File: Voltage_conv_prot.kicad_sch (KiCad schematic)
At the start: 6 parts, among them Q1 AO3400A, U6 MIC5504-3.3YM5-TR

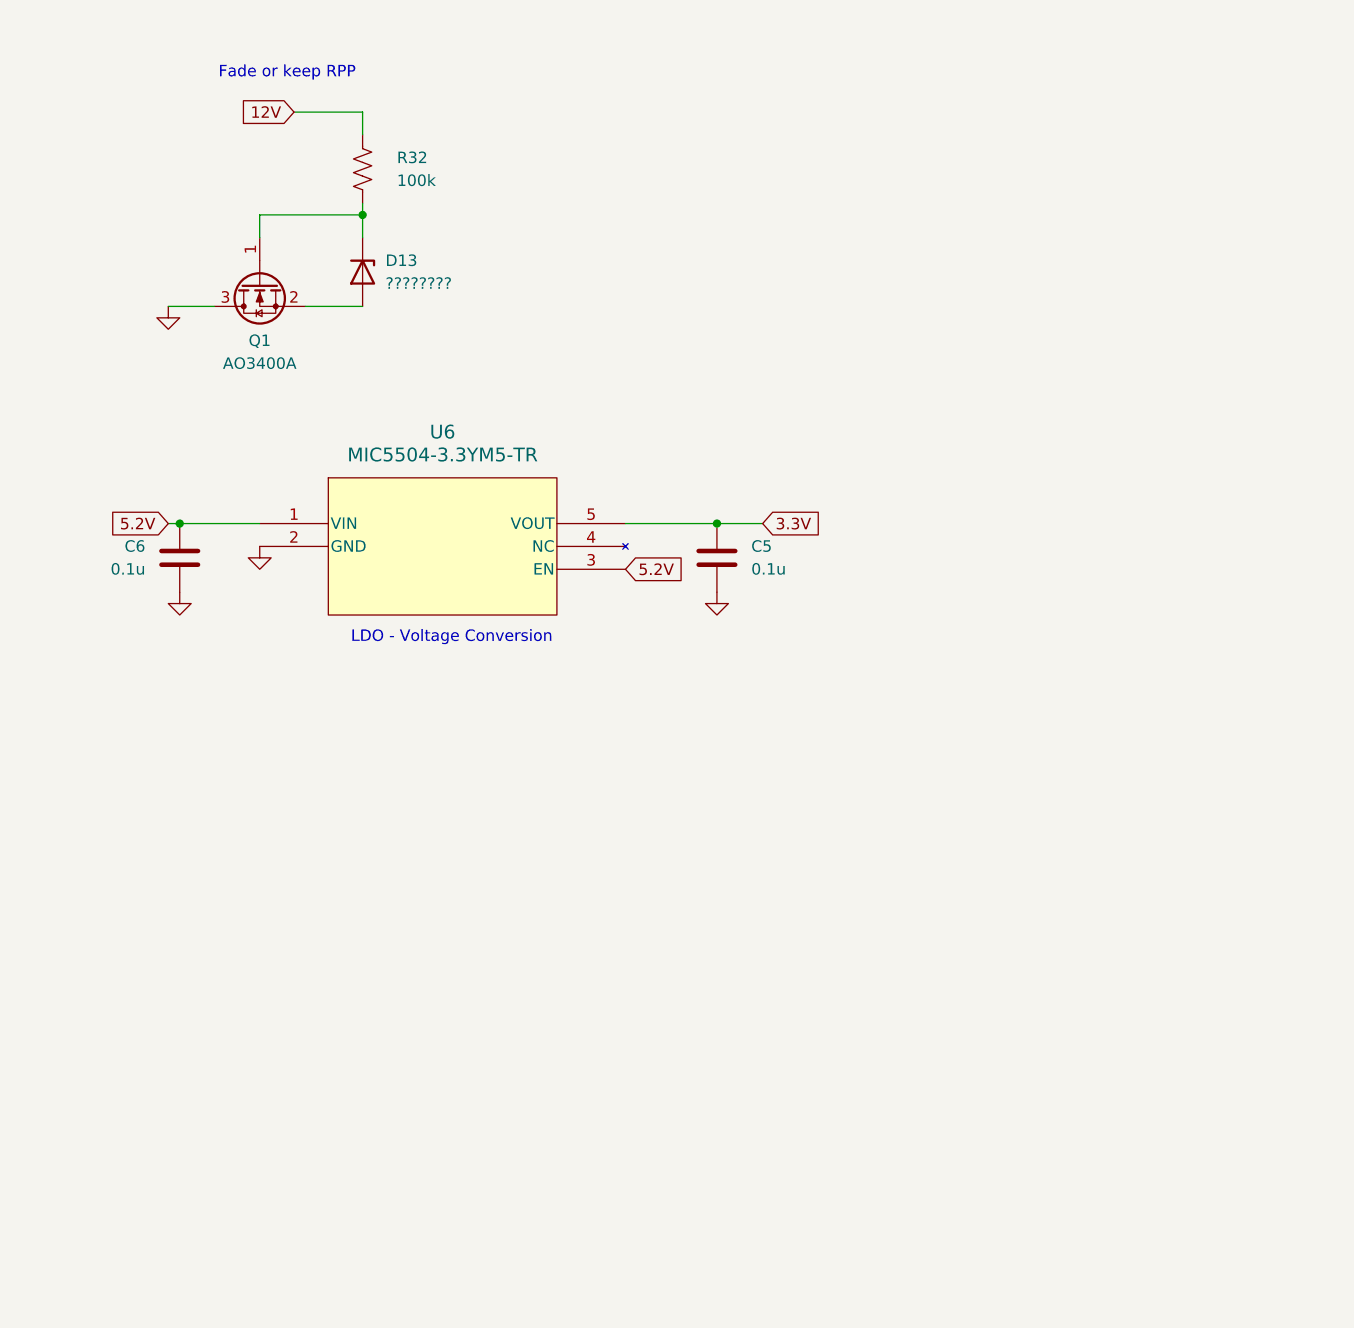
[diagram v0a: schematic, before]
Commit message: Final v1
Finished making it look nice, looking for feedback
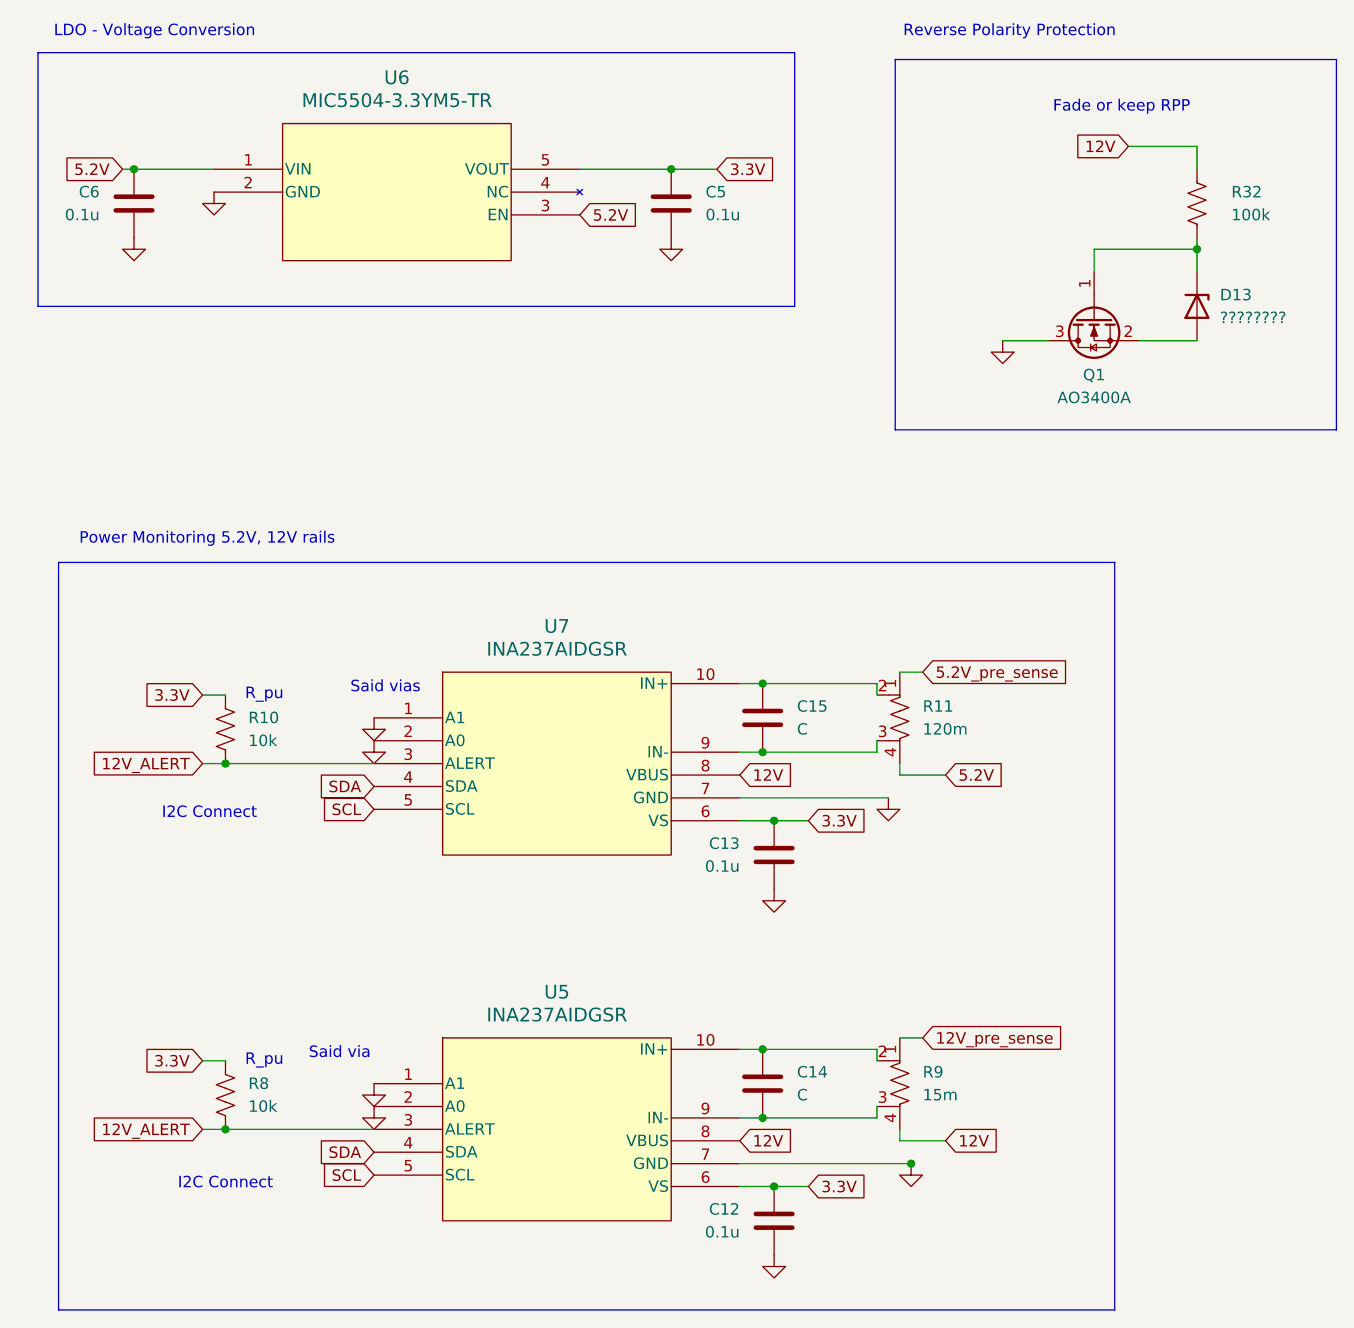
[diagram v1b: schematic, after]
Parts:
- added C12, C13: 0.1u, symbol Device:C
- added C14, C15: C, symbol Device:C
- added R10, R8: 10k, symbol Device:R_US
- added R11: 120m, symbol Device:R_Shunt_US
- added R9: 15m, symbol Device:R_Shunt_US
- added U5, U7: INA237AIDGSR, VSSOP_IDGSR_TEX, symbol board_control_manual_lib:INA237AIDGSR
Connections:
- net 12V: now also R9.4, U5.8 (VBUS), U7.8 (VBUS)
- net 3.3V: now also C12.1, C13.1, R10.1, R8.1, U5.6 (VS), U7.6 (VS)
- net 5.2V: now also R11.4
- net GND: now also C12.2, C13.2, U5.1 (A1), U5.2 (A0), U5.7 (GND), U7.1 (A1), U7.2 (A0), U7.7 (GND)
- new net: C15.1, R11.2, U7.10 (IN+)
- new net: C15.2, R11.3, U7.9 (IN-)
- new net: C14.1, R9.2, U5.10 (IN+)
- new net: C14.2, R9.3, U5.9 (IN-)
- new net 12V_ALERT: R10.2, R8.2, U5.3 (ALERT), U7.3 (ALERT)
- new net 12V_pre_sense: R9.1
- new net 5.2V_pre_sense: R11.1
- new net SCL: U5.5 (SCL), U7.5 (SCL)
- new net SDA: U5.4 (SDA), U7.4 (SDA)
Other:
- note added: "I2C Connect"
- note added: "Power Monitoring 5.2V, 12V rails"
- note added: "R_pu"
- note added: "Reverse Polarity Protection"
- note added: "Said via"
- note added: "Said vias"
- moved on the sheet: C5, C6, D13, Q1, R32, U6
